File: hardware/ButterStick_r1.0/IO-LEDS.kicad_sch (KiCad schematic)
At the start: 20 parts, among them Q1 Q_NMOS_GSD, Q2 Q_NMOS_GSD, Q3 Q_NMOS_GSD

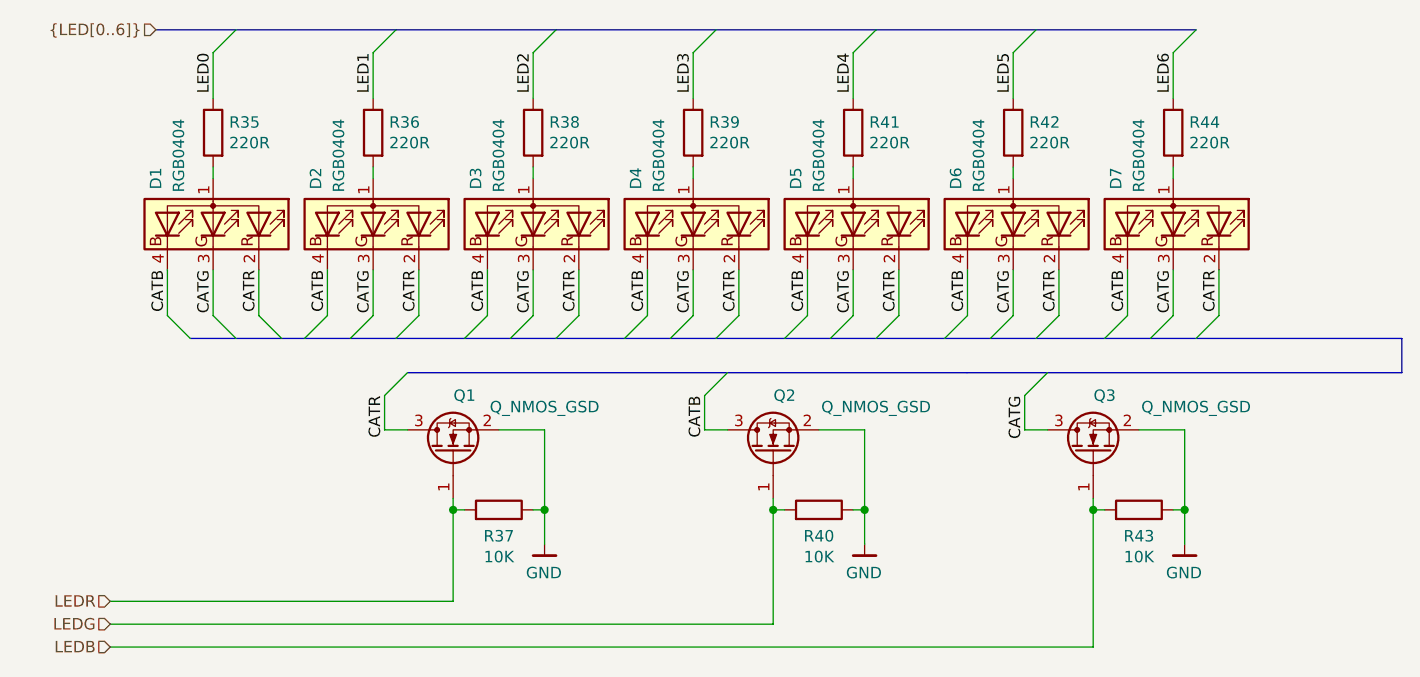
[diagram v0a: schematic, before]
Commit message: hw.r1d0: Review complete, gerbers generated
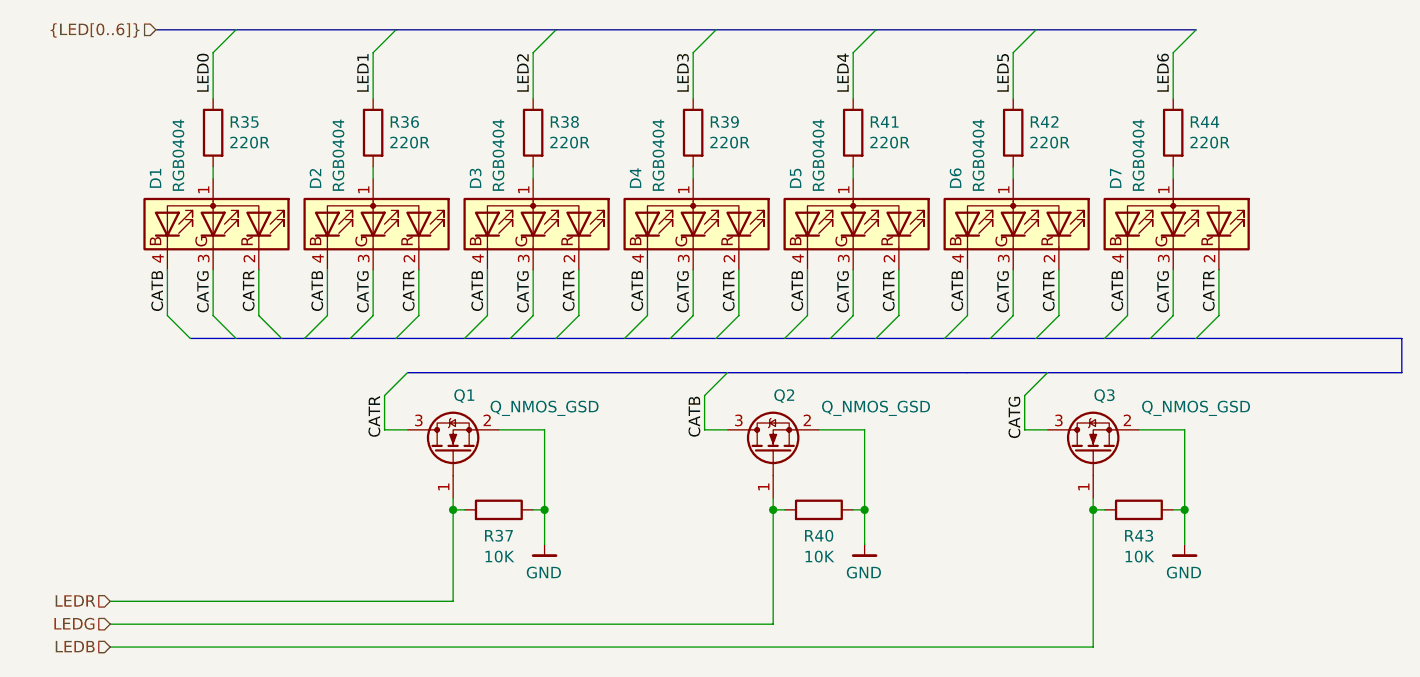
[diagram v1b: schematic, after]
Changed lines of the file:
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@@
 (kicad_sch (version 20200618) (host eeschema "5.99.0-unknown-73168a9~101~ubuntu18.04.1")
-  (page 1 18)
+  (page 5 18)
   (paper "A4")
   (title_block
     (title "ButterStick")
-    (date "2020-07-16")
+    (date "2020-07-17")
     (rev "r1.0")
     (company "GsD")
@@
     (stroke (width 0) (type solid) (color 0 0 0 0))
   )
-  (bus (pts (xy 110.49 106.68) (xy 118.11 106.68))
+  (bus (pts (xy 110.49 106.68) (xy 123.19 106.68))
     (stroke (width 0) (type solid) (color 0 0 0 0))
   )
@@
     (stroke (width 0) (type solid) (color 0 0 0 0))
   )
-  (bus (pts (xy 118.11 106.68) (xy 128.27 106.68))
+  (bus (pts (xy 123.19 106.68) (xy 128.27 106.68))
     (stroke (width 0) (type solid) (color 0 0 0 0))
   )
@@
     (stroke (width 0) (type solid) (color 0 0 0 0))
   )
-  (bus (pts (xy 128.27 106.68) (xy 135.89 106.68))
-    (stroke (width 0) (type solid) (color 0 0 0 0))
-  )
-  (bus (pts (xy 135.89 106.68) (xy 146.05 106.68))
-    (stroke (width 0) (type solid) (color 0 0 0 0))
-  )
-  (bus (pts (xy 146.05 106.68) (xy 158.75 106.68))
-    (stroke (width 0) (type solid) (color 0 0 0 0))
-  )
-  (bus (pts (xy 158.75 106.68) (xy 171.45 106.68))
+  (bus (pts (xy 128.27 106.68) (xy 140.97 106.68))
+    (stroke (width 0) (type solid) (color 0 0 0 0))
+  )
+  (bus (pts (xy 140.97 106.68) (xy 153.67 106.68))
+    (stroke (width 0) (type solid) (color 0 0 0 0))
+  )
+  (bus (pts (xy 153.67 106.68) (xy 163.83 106.68))
     (stroke (width 0) (type solid) (color 0 0 0 0))
   )
@@
     (stroke (width 0) (type solid) (color 0 0 0 0))
   )
-  (bus (pts (xy 171.45 106.68) (xy 181.61 106.68))
+  (bus (pts (xy 163.83 106.68) (xy 176.53 106.68))
     (stroke (width 0) (type solid) (color 0 0 0 0))
   )
@@
     (stroke (width 0) (type solid) (color 0 0 0 0))
   )
-  (bus (pts (xy 181.61 106.68) (xy 194.31 106.68))
-    (stroke (width 0) (type solid) (color 0 0 0 0))
-  )
+  (bus (pts (xy 176.53 106.68) (xy 189.23 106.68))
+    (stroke (width 0) (type solid) (color 0 0 0 0))
+  )
+  (bus (pts (xy 189.23 106.68) (xy 194.31 106.68))
+    (stroke (width 0) (type solid) (color 0 0 0 0))
+  )
